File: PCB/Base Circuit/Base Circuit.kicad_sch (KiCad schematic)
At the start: 0 parts

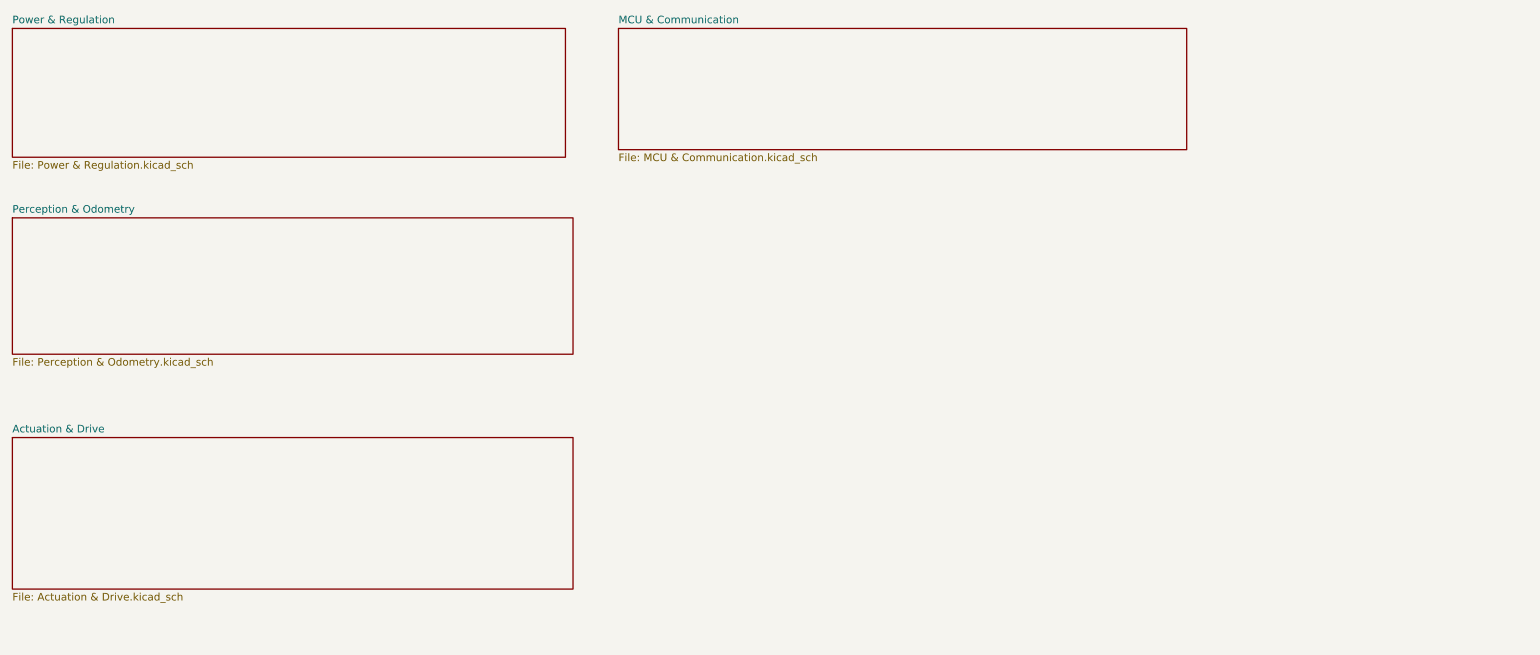
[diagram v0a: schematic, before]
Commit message: PCB Updated
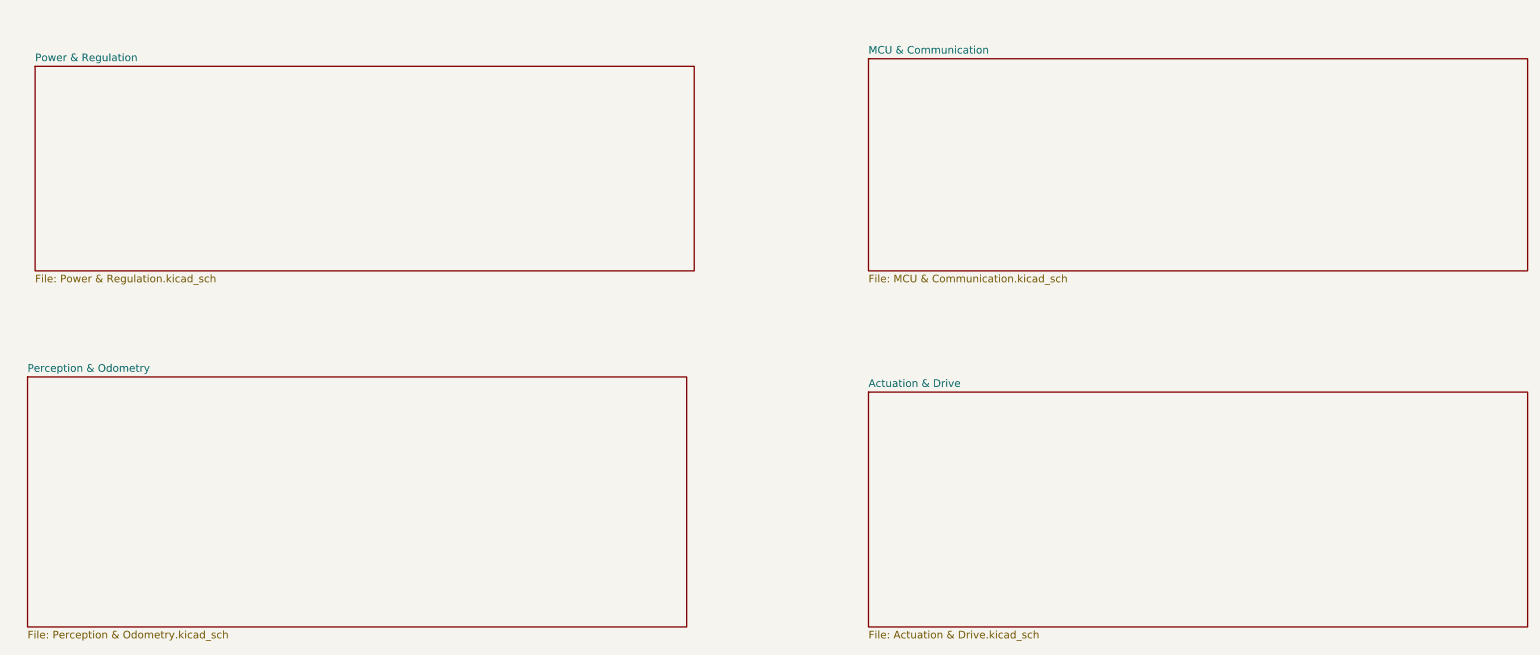
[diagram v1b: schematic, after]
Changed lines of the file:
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@@
 	(paper "A4")
 	(sheet
-		(at 20.32 21.59)
-		(size 92.71 21.59)
+		(at 24.13 27.94)
+		(size 110.49 34.29)
 		(exclude_from_sim no)
 		(in_bom yes)
@@
 		)
 		(property "Sheetname" "Power & Regulation"
-			(at 20.32 20.8784 0)
+			(at 24.13 27.2284 0)
 			(effects
 				(font
@@
 		)
 		(property "Sheetfile" "Power & Regulation.kicad_sch"
-			(at 20.32 43.7646 0)
+			(at 24.13 62.8146 0)
 			(effects
 				(font
@@
 	)
 	(sheet
-		(at 20.32 90.17)
-		(size 93.98 25.4)
+		(at 163.83 82.55)
+		(size 110.49 39.37)
 		(exclude_from_sim no)
 		(in_bom yes)
@@
 		)
 		(property "Sheetname" "Actuation & Drive"
-			(at 20.32 89.4584 0)
+			(at 163.83 81.8384 0)
 			(effects
 				(font
@@
 		)
 		(property "Sheetfile" "Actuation & Drive.kicad_sch"
-			(at 20.32 116.1546 0)
+			(at 163.83 122.5046 0)
 			(effects
 				(font
@@
 	)
 	(sheet
-		(at 121.92 21.59)
-		(size 95.25 20.32)
+		(at 163.83 26.67)
+		(size 110.49 35.56)
 		(exclude_from_sim no)
 		(in_bom yes)
@@
 		)
 		(property "Sheetname" "MCU & Communication"
-			(at 121.92 20.8784 0)
+			(at 163.83 25.9584 0)
 			(effects
 				(font
@@
 		)
 		(property "Sheetfile" "MCU & Communication.kicad_sch"
-			(at 121.92 42.4946 0)
+			(at 163.83 62.8146 0)
 			(effects
 				(font
@@
 	)
 	(sheet
-		(at 20.32 53.34)
-		(size 93.98 22.86)
+		(at 22.86 80.01)
+		(size 110.49 41.91)
 		(exclude_from_sim no)
 		(in_bom yes)
@@
 		)
 		(property "Sheetname" "Perception & Odometry"
-			(at 20.32 52.6284 0)
+			(at 22.86 79.2984 0)
 			(effects
 				(font
@@
 		)
 		(property "Sheetfile" "Perception & Odometry.kicad_sch"
-			(at 20.32 76.7846 0)
+			(at 22.86 122.5046 0)
 			(effects
 				(font
